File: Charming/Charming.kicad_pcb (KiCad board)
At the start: 2 copper layers, 29 parts, among them J1 AVR ISP, SW1 SW_Push, SW2 SW_Push, SW3 SW_Push, SW4 SW_Push, U1 ATmega328P-PU, Y1 16MHz

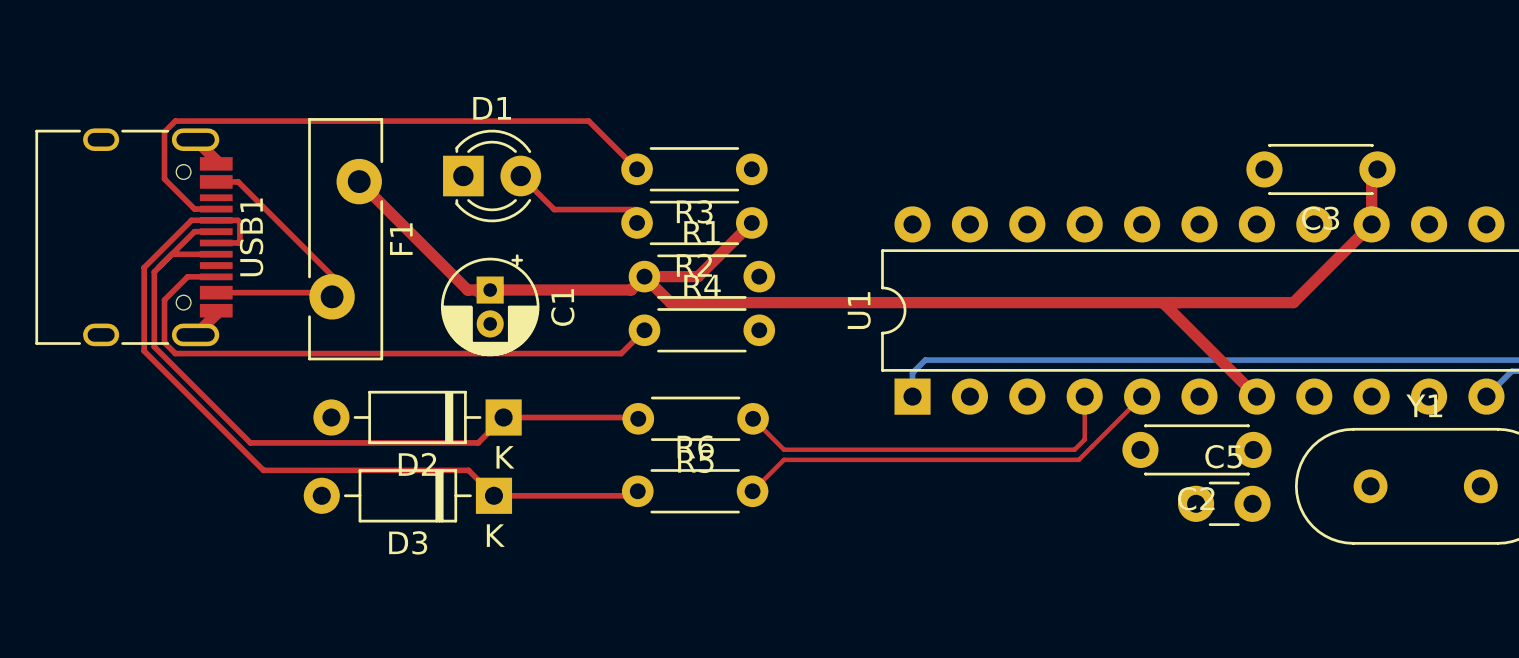
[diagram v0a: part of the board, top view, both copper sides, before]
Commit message: name netlist
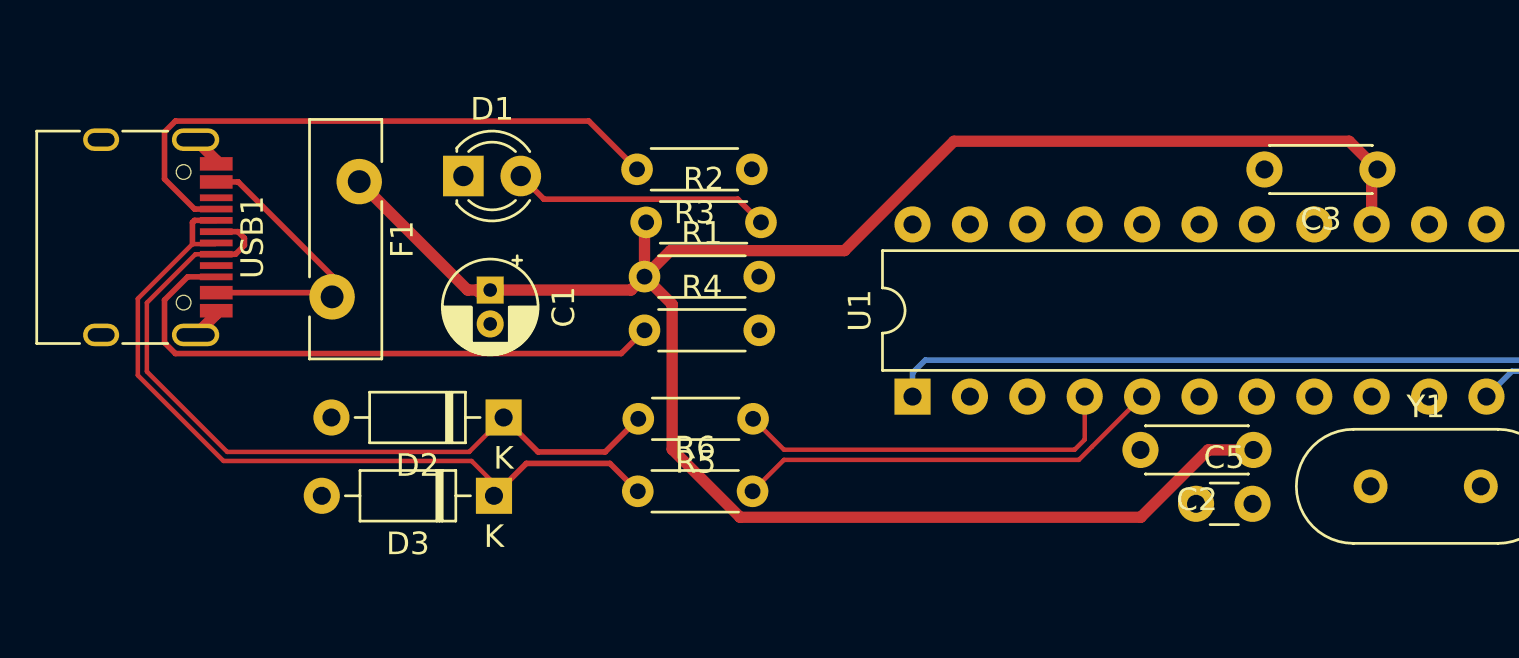
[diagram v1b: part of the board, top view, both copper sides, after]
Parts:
- moved R2 4.68 mm to (58.8, 87.7), turned to 0 degrees
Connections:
- net Net-(D2-Pad1) renamed /DP
- net Net-(D3-Pad1) renamed /DN
- net Net-(F1-Pad2) renamed /VSUB
- net Net-(R3-Pad2) renamed /CC1
- net Net-(R4-Pad1) renamed /CC2
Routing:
- net +5V: track 64.3 -> 92.0 mm
- net Net-(D1-Pad2): track 5.76 -> 11.5 mm
- net /DP: track 33.2 -> 35.4 mm

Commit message: move customize footprints to external libs
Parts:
- J1: footprint Charming:AVRISP -> JSA:AVRISP
- USB1: footprint Charming:USB_C_Receptacle_HRO_TYPE-C-31-M-12 -> JSA:USB_C_Receptacle_HRO_TYPE-C-31-M-12
